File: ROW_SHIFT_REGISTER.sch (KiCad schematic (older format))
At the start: 16 parts, among them U12 74HC595, U13 74HC595, U14 74HC595, U15 74HC595

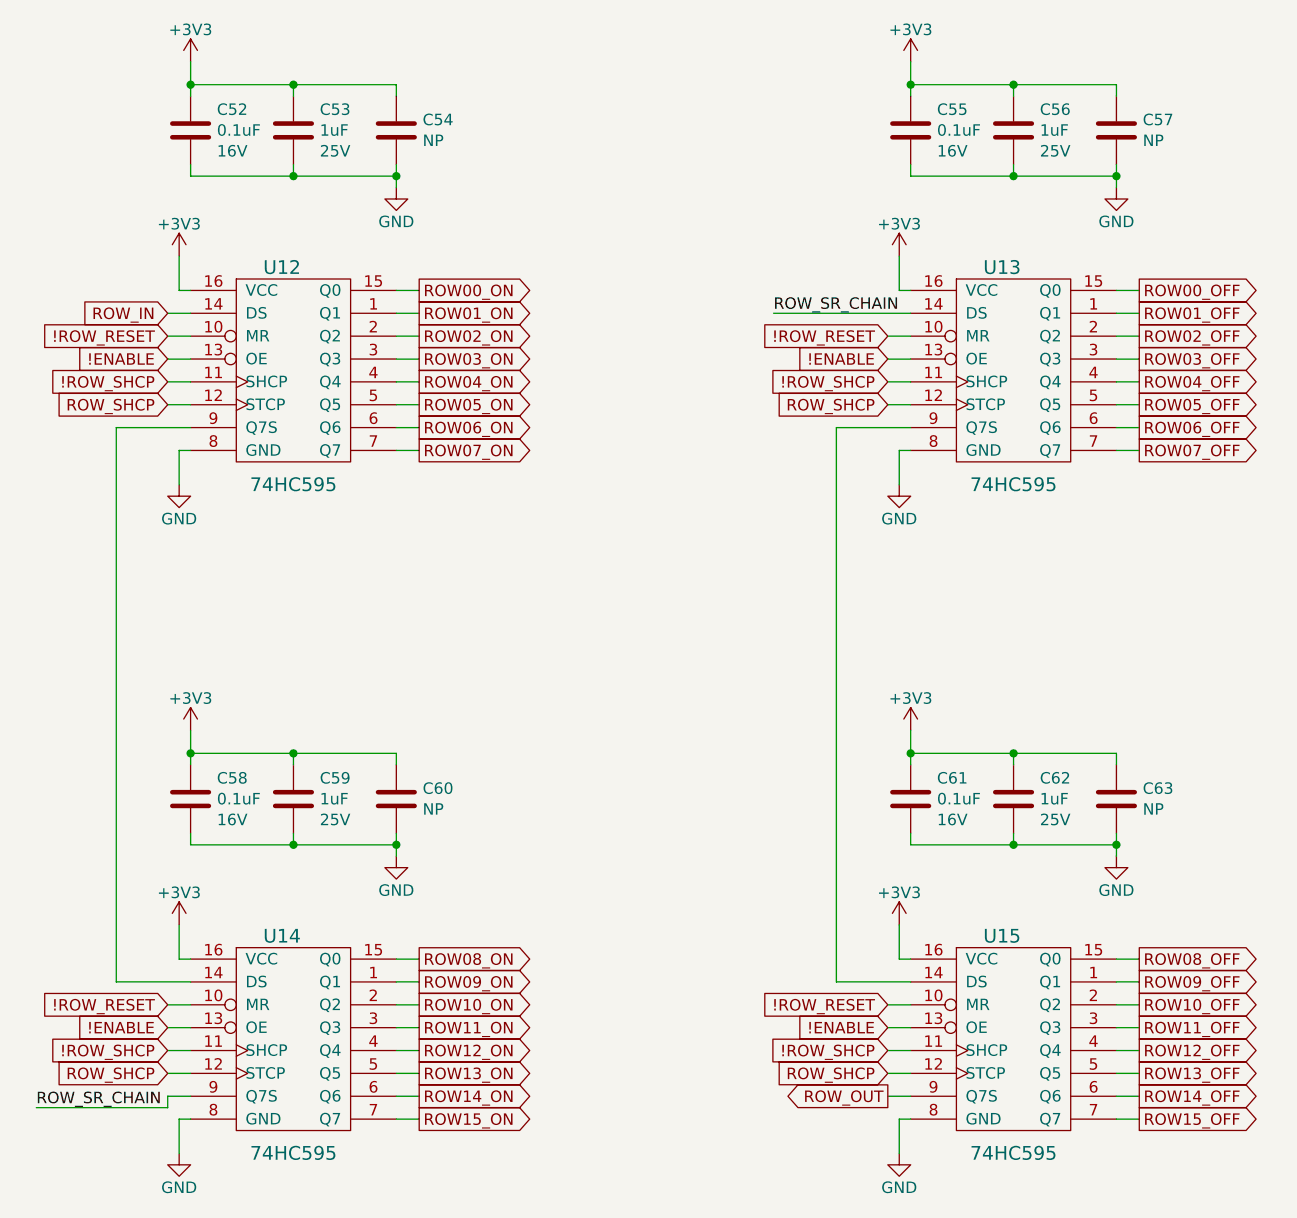
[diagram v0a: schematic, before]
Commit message: automated commit
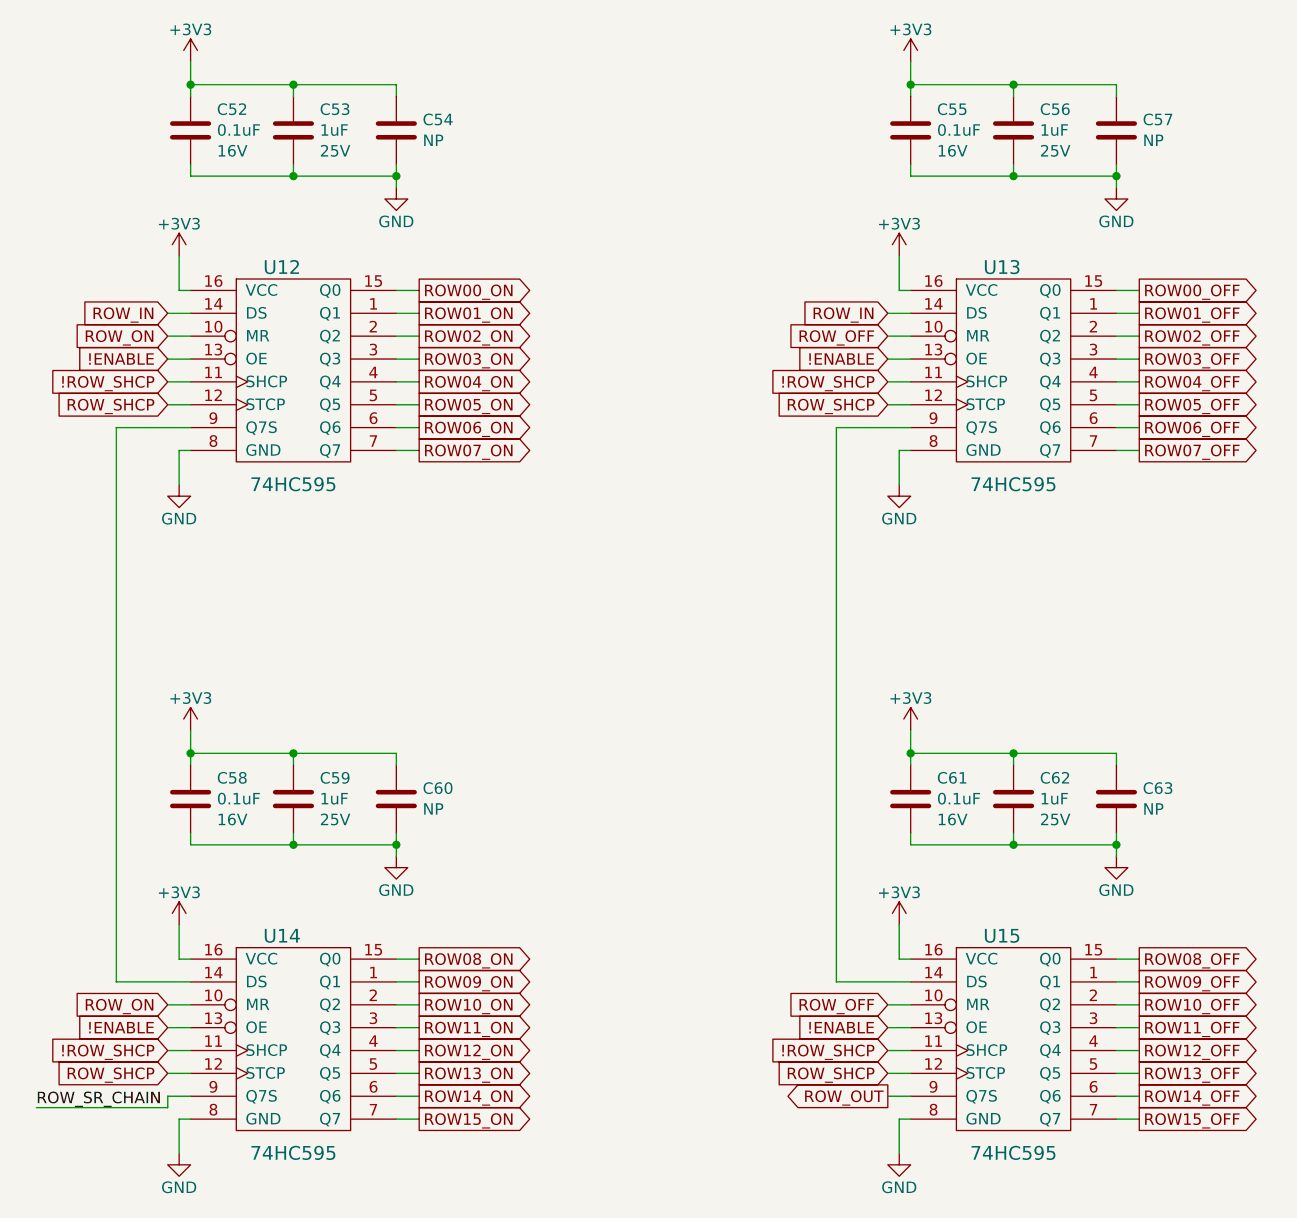
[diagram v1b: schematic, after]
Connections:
- net ROW_IN: now also U13.14 (DS)
- net ROW_SR_CHAIN: no longer U13.14 (DS)
- net !ROW_RESET renamed ROW_OFF
- net ROW_OFF: no longer U12.10 (MR), U14.10 (MR)
- new net ROW_ON: U12.10 (MR), U14.10 (MR)
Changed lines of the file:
@@
 F 1 "74HC595" H 5525 2100 60  0000 C CNN
 F 2 "" H 5225 2650 60  0001 C CNN
-F 3 "" H 5225 2650 60  0001 C CNN
+F 3 "~/datasheets/74HC_HCT595.pdf" H 5225 2650 60  0001 C CNN
 	1    5525 2600
 	1    0    0    -1
@@
 Wire Wire Line
 	1825 5775 1925 5775
-Text Label 4475 2350 0    50   ~ 0
-ROW_SR_CHAIN
-Wire Wire Line
-	4475 2350 5075 2350
-Text GLabel 1825 2450 0    50   Input ~ 0
-!ROW_RESET
 Text GLabel 1825 2550 0    50   Input ~ 0
 !ENABLE
@@
 Text GLabel 1825 2750 0    50   Input ~ 0
 ROW_SHCP
-Text GLabel 1825 5375 0    50   Input ~ 0
-!ROW_RESET
 Text GLabel 1825 5475 0    50   Input ~ 0
 !ENABLE
@@
 Text GLabel 1825 5675 0    50   Input ~ 0
 ROW_SHCP
-Text GLabel 4975 2450 0    50   Input ~ 0
-!ROW_RESET
 Text GLabel 4975 2550 0    50   Input ~ 0
 !ENABLE
@@
 Text GLabel 4975 2750 0    50   Input ~ 0
 ROW_SHCP
-Text GLabel 4975 5375 0    50   Input ~ 0
-!ROW_RESET
 Text GLabel 4975 5475 0    50   Input ~ 0
 !ENABLE
@@
 Text GLabel 6075 2950 2    50   Output ~ 0
 ROW07_OFF
+Wire Wire Line
+	5075 2350 4975 2350
+Text GLabel 4975 2350 0    50   Input ~ 0
+ROW_IN
+Text GLabel 1825 5375 0    50   Input ~ 0
+ROW_ON
+Text GLabel 1825 2450 0    50   Input ~ 0
+ROW_ON
+Text GLabel 4975 2450 0    50   Input ~ 0
+ROW_OFF
+Text GLabel 4975 5375 0    50   Input ~ 0
+ROW_OFF
 $EndSCHEMATC
